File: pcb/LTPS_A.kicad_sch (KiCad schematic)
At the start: 0 parts

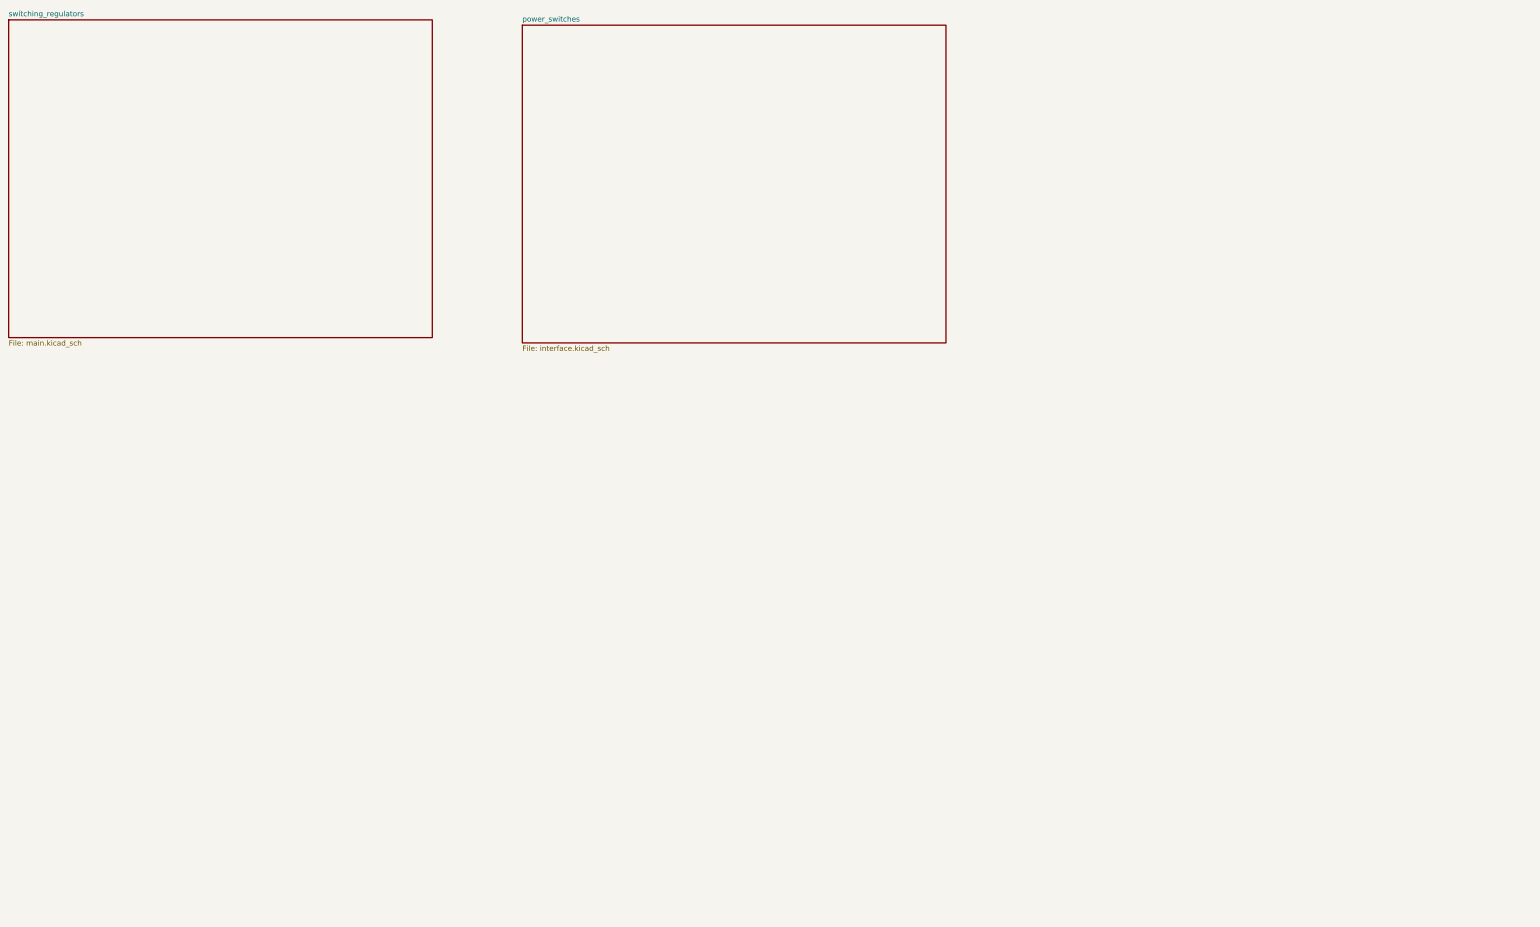
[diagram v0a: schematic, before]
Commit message: fixed license
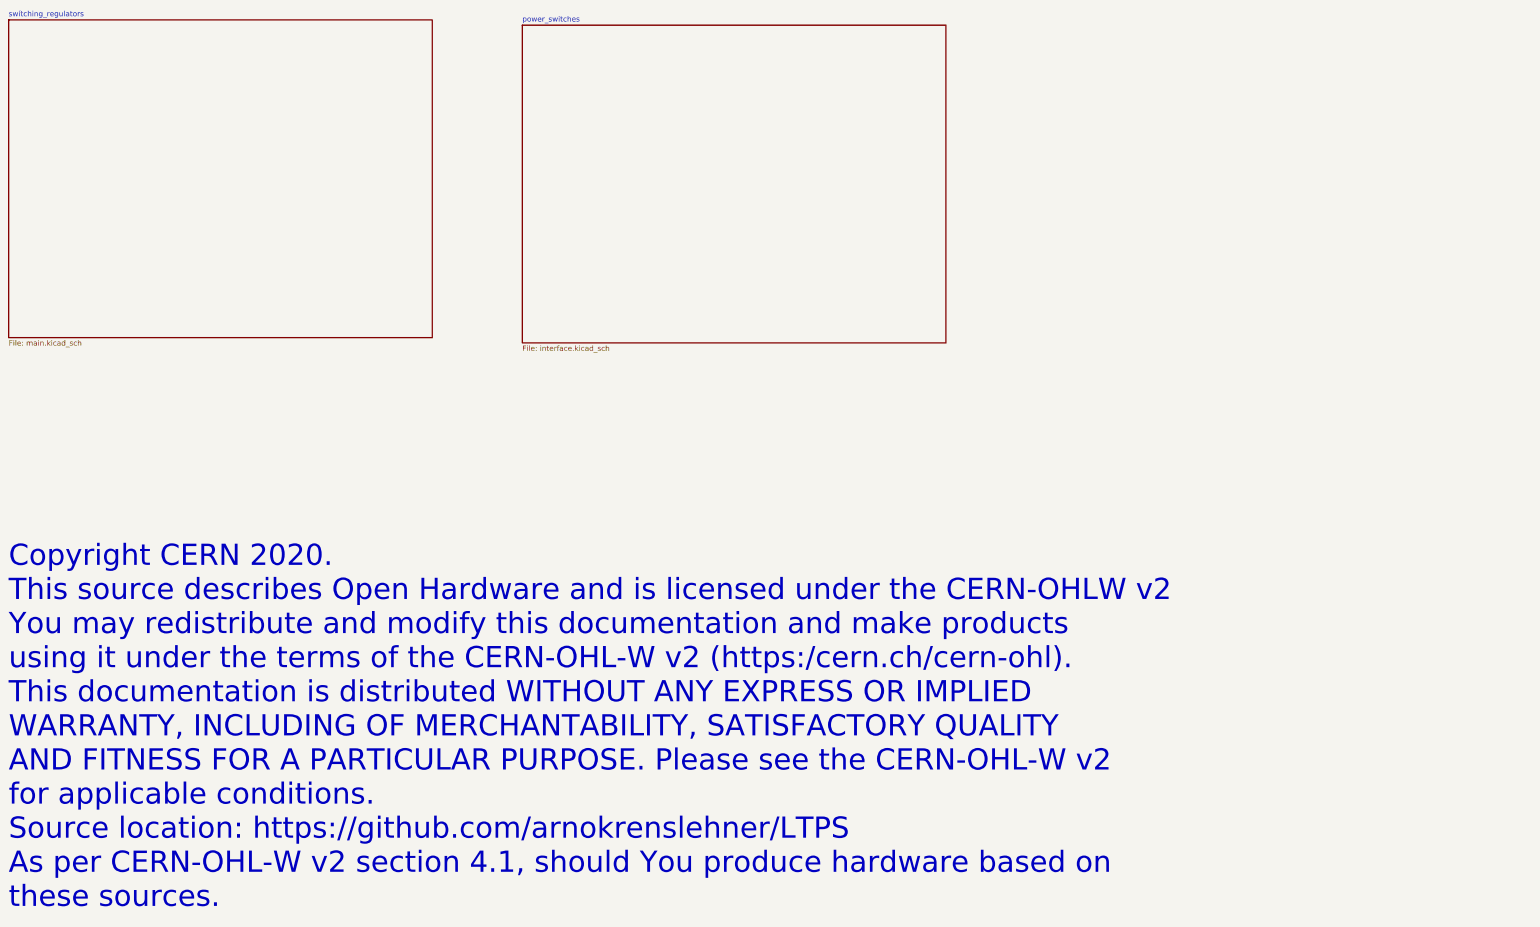
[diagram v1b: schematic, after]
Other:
- note added: "Copyright CERN 2020. This source describes Open Hardware and is licensed under the CERN-OHLW v2 You may redistribute and modify this documentation and make products using it under the terms of the CERN-OHL-W v2 (https:/cern.ch/cern-ohl). This documentation is distributed WITHOUT ANY EXPRESS OR IMPLIED WARRANTY, INCLUDING OF MERCHANTABILITY, SATISFACTORY QUALITY AND FITNESS FOR A PARTICULAR PURPOS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"
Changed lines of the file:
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@@
     (comment 4 "en")
+  )
+  (text "Copyright CERN 2020.\nThis source describes Open Hardware and is licensed under the CERN-OHLW v2\nYou may redistribute and modify this documentation and make products\nusing it under the terms of the CERN-OHL-W v2 (https:/cern.ch/cern-ohl).\nThis documentation is distributed WITHOUT ANY EXPRESS OR IMPLIED\nWARRANTY, INCLUDING OF MERCHANTABILITY, SATISFACTORY QUALITY\nAND FITNESS FOR A PARTICULAR PURPOSE. Please see the CERN-OHL-W v2\nfor applicable conditions.\nSource location: https://github.com/arnokrenslehner/LTPS\nAs per CERN-OHL-W v2 section 4.1, should You produce hardware based on\nthese sources."
+    (at 39.37 238.76 0)
+    (effects (font (size 5.08 5.08)) (justify left bottom))
   )
   (sheet (at 162.56 26.67) (size 101.6 76.2) (fields_autoplaced)
